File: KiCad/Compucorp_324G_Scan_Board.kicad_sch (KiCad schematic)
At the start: 24 parts, among them J1 Scan Interboard, J2 Power In, J4 From Keyboard, U1 BR 16252, U2 UHP480, U21 TMC1884 (TCL08), U3 UHP480, U4 TMC1869 (TCL02)

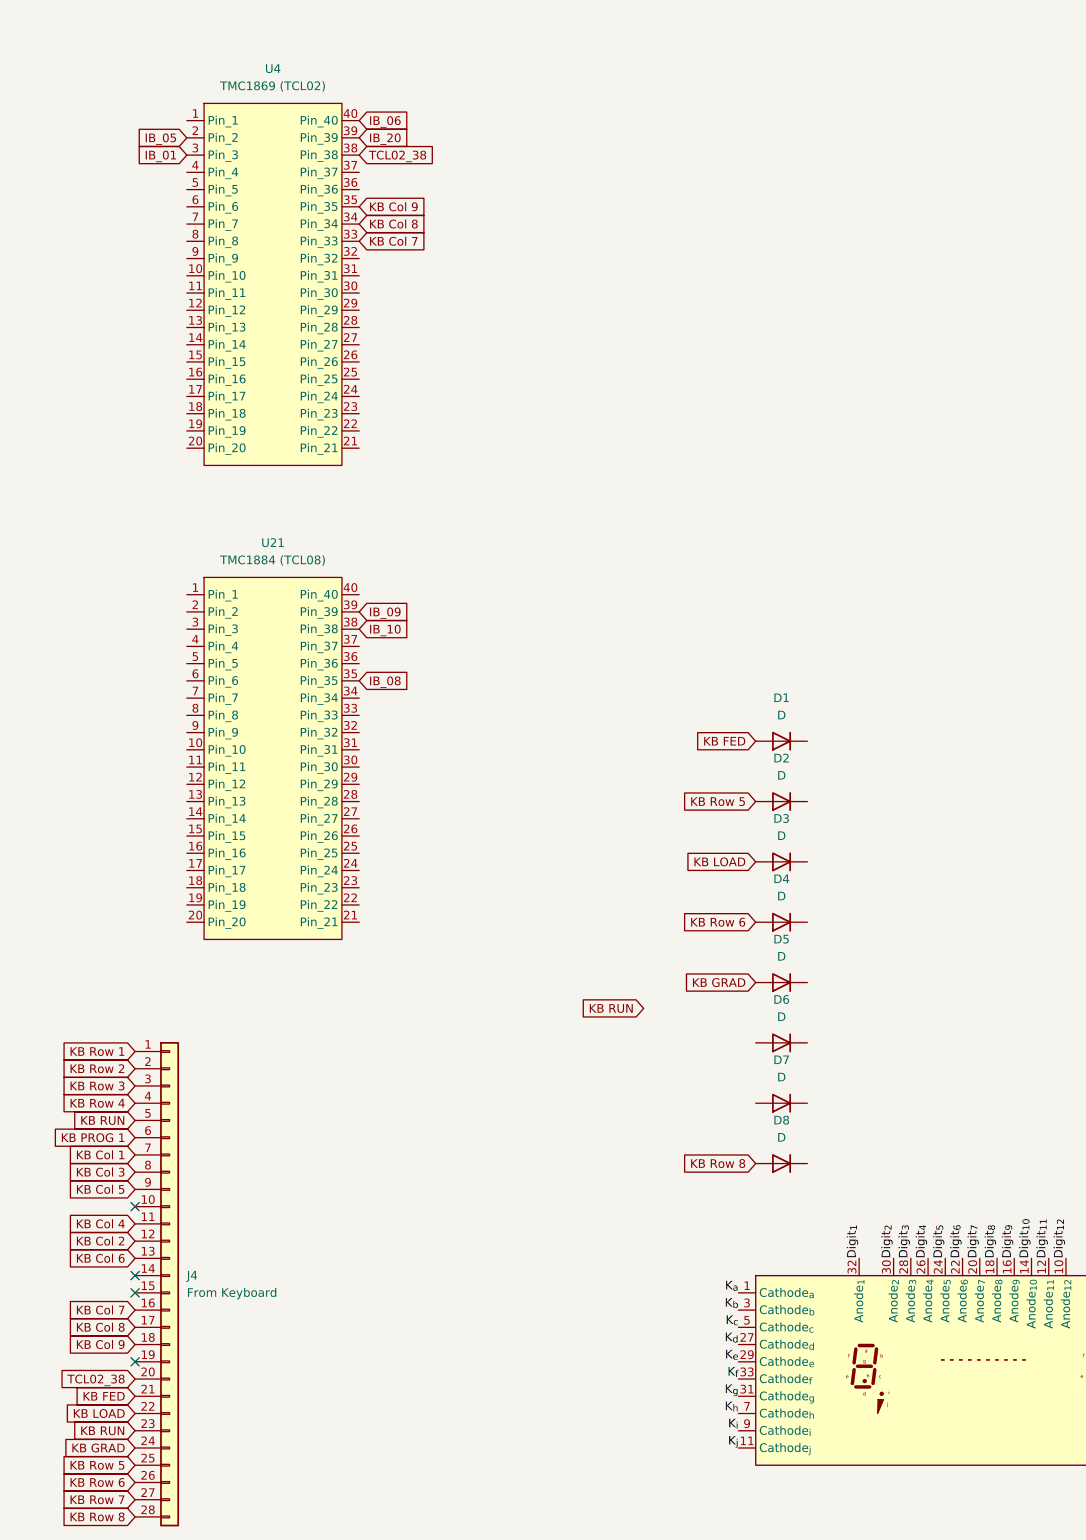
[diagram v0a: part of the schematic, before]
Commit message: Update Compucorp_324G_Scan_Board.kicad_sch
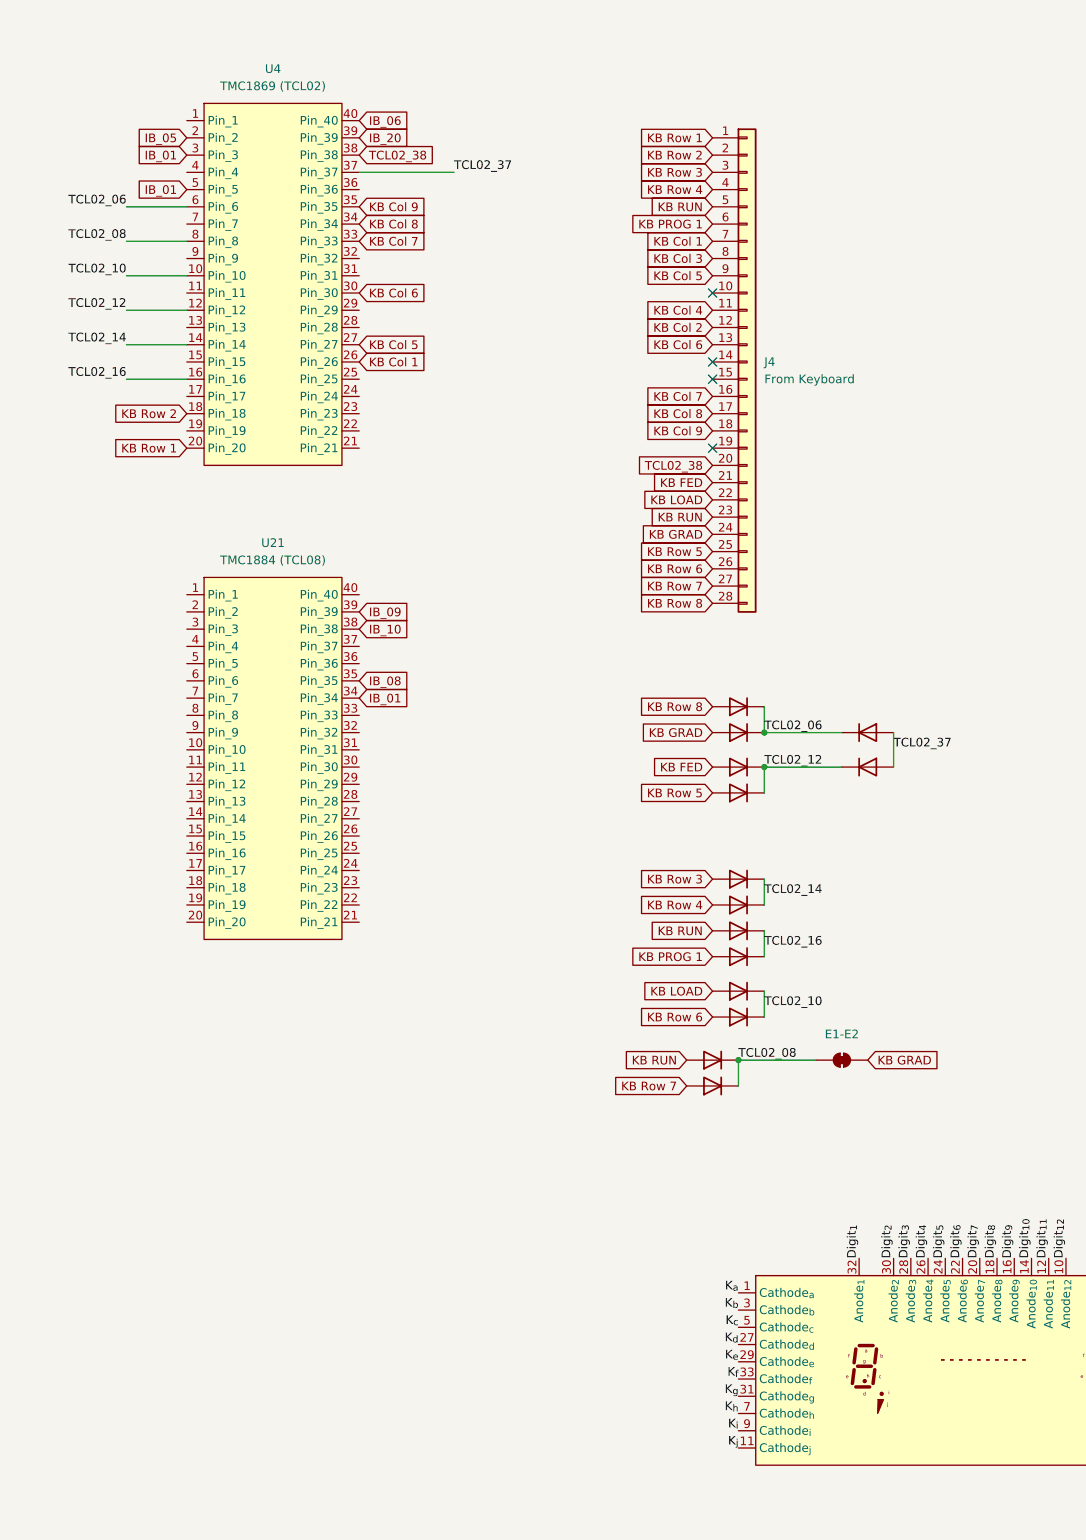
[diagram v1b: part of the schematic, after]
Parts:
- added D13, D14, D15, D16, D17, D18: D, symbol Device:D
- added JP1: E1-E2, symbol Jumper:SolderJumper_2_Bridged
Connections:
- net IB_01: now also U21.34 (Pin_34), U4.5 (Pin_5)
- net KB Col 1: now also U4.26 (Pin_26)
- net KB Col 5: now also U4.27 (Pin_27)
- net KB Col 6: now also U4.30 (Pin_30)
- net KB GRAD: now also JP1.2 (B)
- net KB PROG 1: now also D15.2 (A)
- net KB RUN: now also D6.2 (A), D13.2 (A)
- net KB Row 1: now also U4.20 (Pin_20)
- net KB Row 2: now also U4.18 (Pin_18)
- net KB Row 3: now also D14.2 (A)
- net KB Row 4: now also D16.2 (A)
- net KB Row 7: now also D7.2 (A)
- net TCL02_10: now reaches D3.1 (K)
- net TCL02_10: now also D4.1 (K), U4.10 (Pin_10)
- net TCL02_06: now reaches D8.1 (K)
- net TCL02_06: now also D5.1 (K), U4.6 (Pin_6), D18.1 (K)
- net TCL02_12: now reaches D2.1 (K)
- net TCL02_12: now also D1.1 (K), U4.12 (Pin_12), D17.1 (K)
- net TCL02_08: now reaches D7.1 (K)
- net TCL02_08: now also D6.1 (K), U4.8 (Pin_8), JP1.1 (A)
- net TCL02_14: now reaches U4.14 (Pin_14)
- net TCL02_14: now also D14.1 (K), D16.1 (K)
- net TCL02_16: now reaches U4.16 (Pin_16)
- net TCL02_16: now also D13.1 (K), D15.1 (K)
- net TCL02_37: now reaches U4.37 (Pin_37)
- net TCL02_37: now also D17.2 (A), D18.2 (A)
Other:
- moved on the sheet: J4
